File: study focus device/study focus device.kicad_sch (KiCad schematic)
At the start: 1 part, among them U1 MCP23017_SP

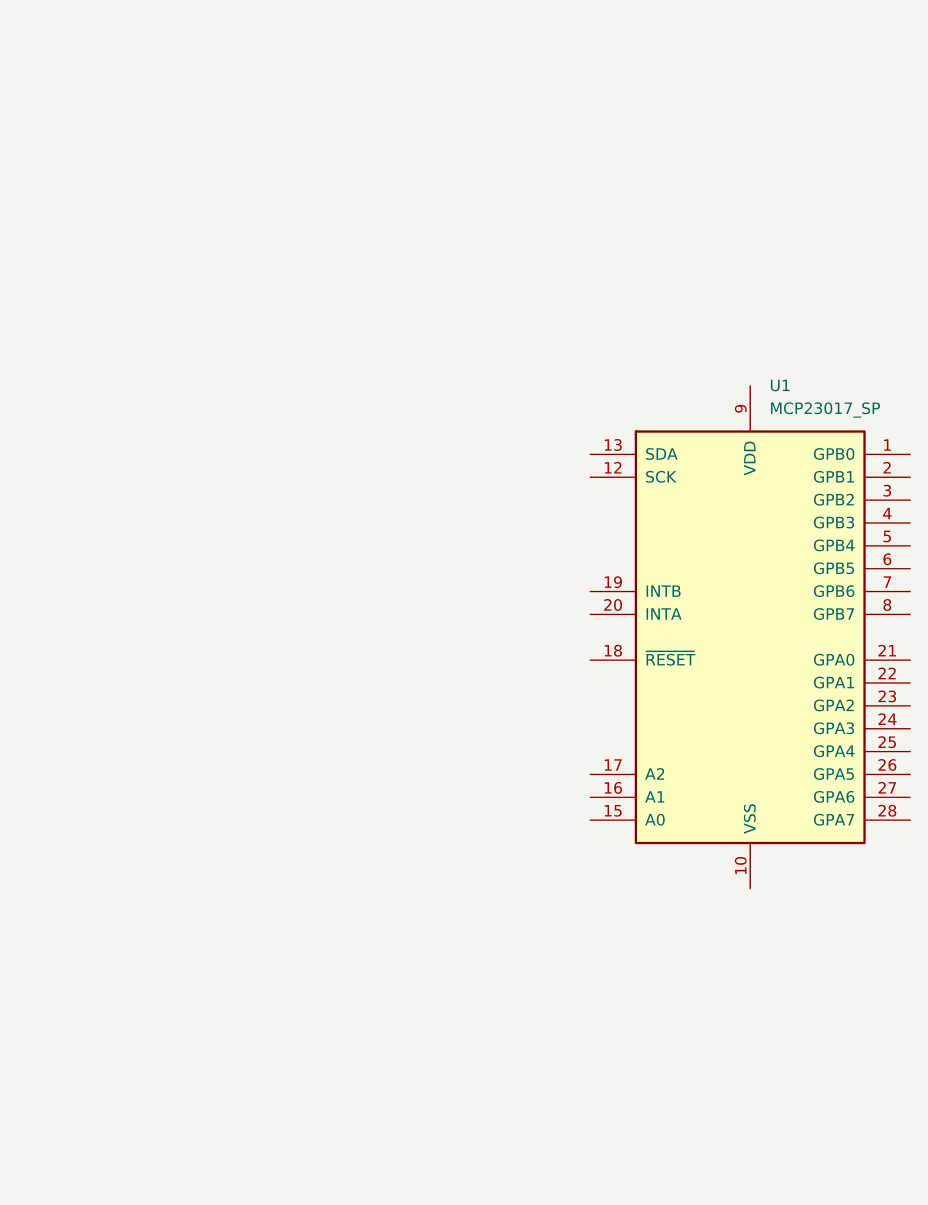
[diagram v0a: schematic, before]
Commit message: more additions
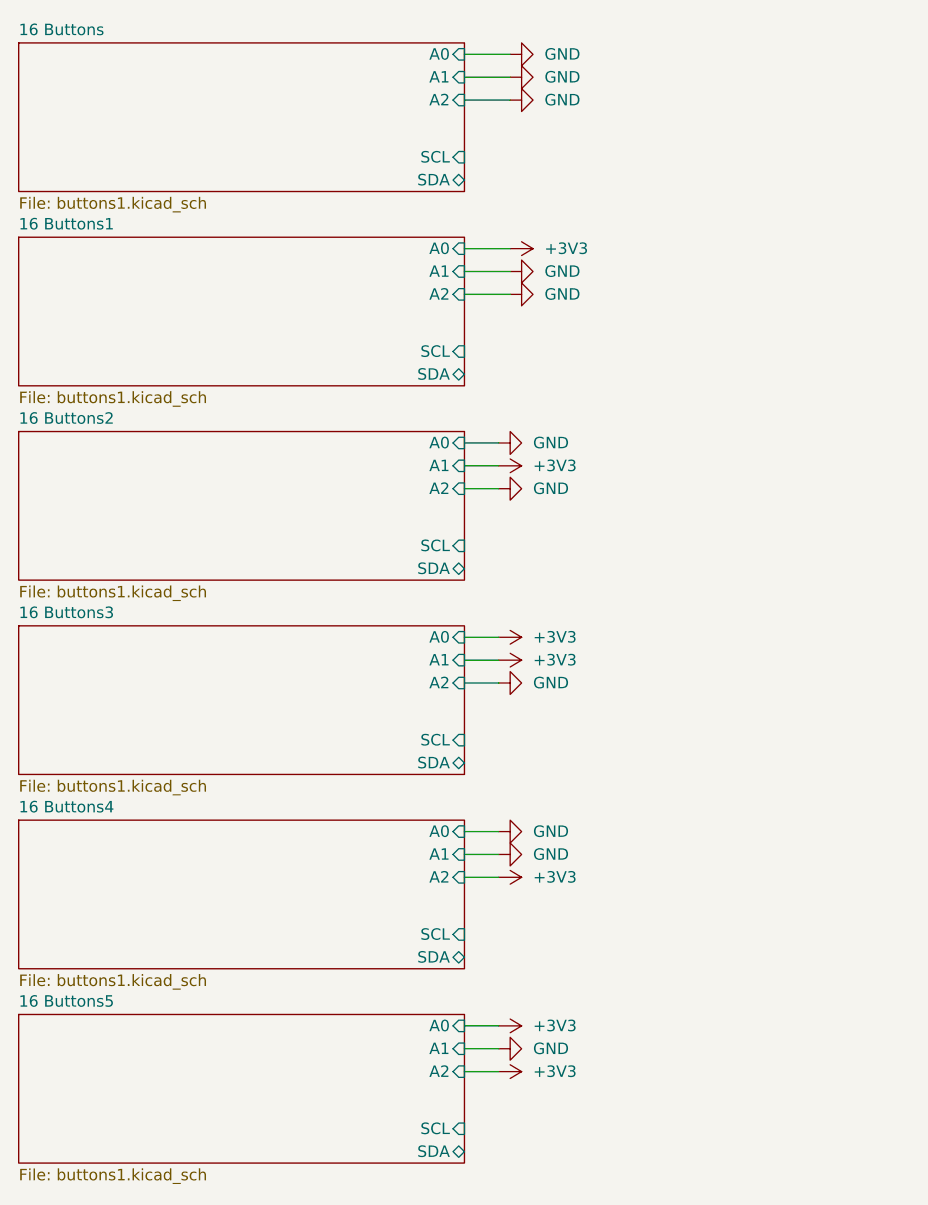
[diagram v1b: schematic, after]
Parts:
- removed U1: MCP23017_SP, Package_DIP:DIP-28_W7.62mm, symbol Interface_Expansion:MCP23017_SP
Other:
- added sheet 16 Buttons (buttons1.kicad_sch)
- added sheet 16 Buttons1 (buttons1.kicad_sch)
- added sheet 16 Buttons2 (buttons1.kicad_sch)
- added sheet 16 Buttons3 (buttons1.kicad_sch)
- added sheet 16 Buttons4 (buttons1.kicad_sch)
- added sheet 16 Buttons5 (buttons1.kicad_sch)
